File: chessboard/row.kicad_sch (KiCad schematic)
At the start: 15 parts, among them U1 PCA9548ADB

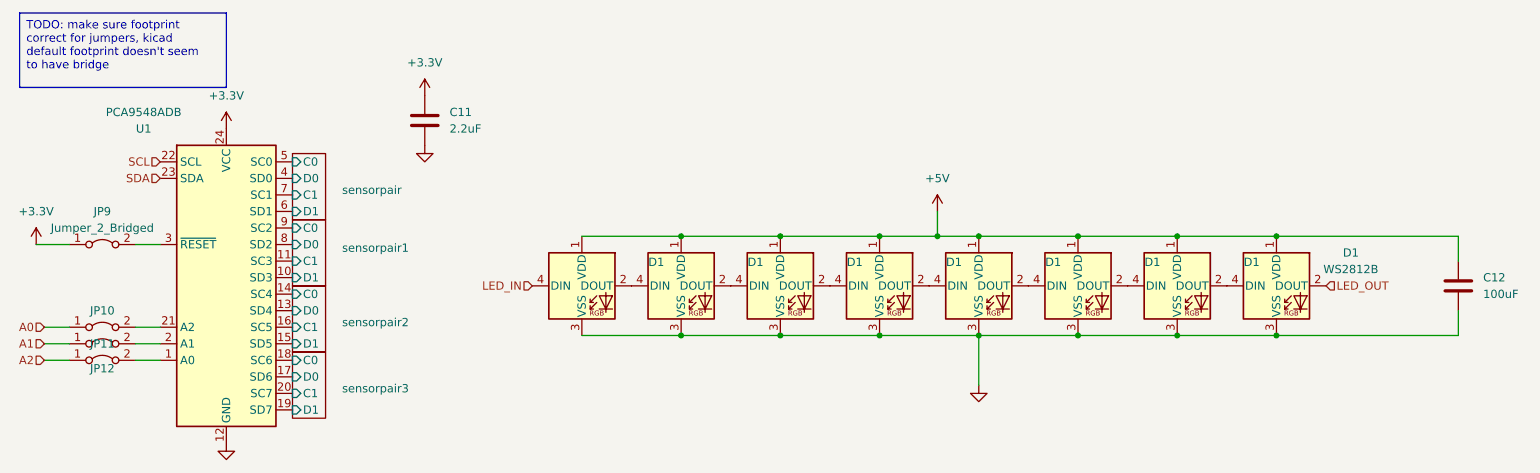
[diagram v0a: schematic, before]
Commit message: a
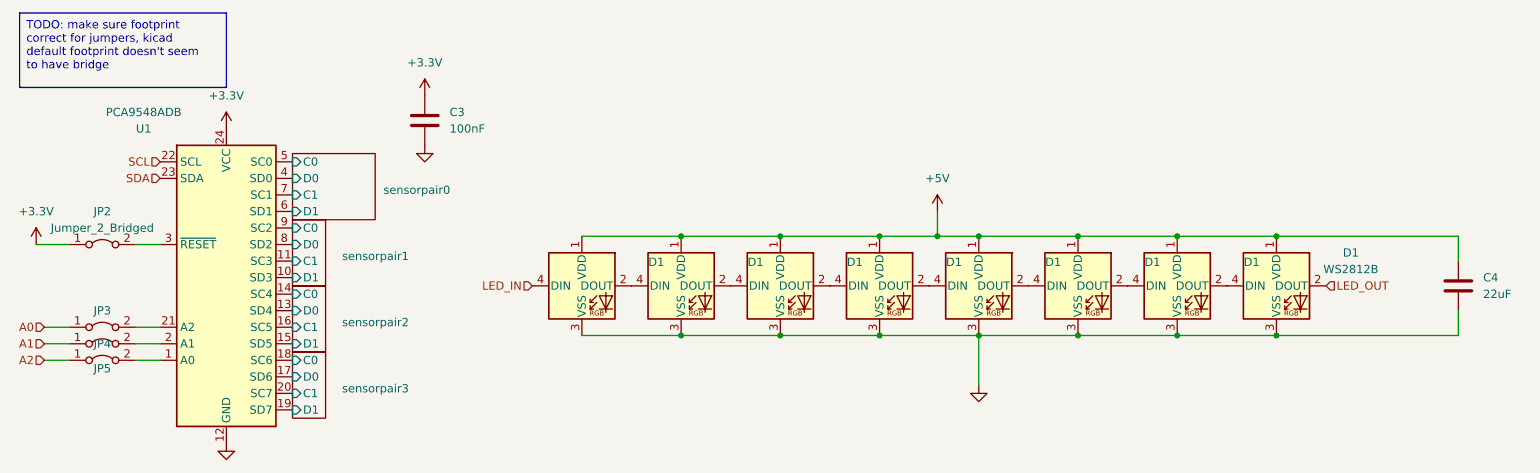
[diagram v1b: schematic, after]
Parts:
- C3: renamed from C11; value 2.2uF -> 100nF; footprint (none) -> Capacitor_SMD:C_0805_2012Metric_Pad1.18x1.45mm_HandSolder
- C4: renamed from C12; value 100uF -> 22uF; footprint (none) -> Capacitor_SMD:C_0805_2012Metric_Pad1.18x1.45mm_HandSolder
- JP2: renamed from JP9; footprint (none) -> mylibrary:Bridged 2.5mm 1.0mm Test Points
- JP3: renamed from JP10; footprint (none) -> mylibrary:Bridged 2.5mm 1.0mm Test Points
- JP4: renamed from JP11; footprint (none) -> mylibrary:Bridged 2.5mm 1.0mm Test Points
- JP5: renamed from JP12; footprint (none) -> mylibrary:Bridged 2.5mm 1.0mm Test Points
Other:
- sheet sensorpair renamed sensorpair0
